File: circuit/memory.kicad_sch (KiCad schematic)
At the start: 26 parts, among them J2 Port C, J3 Port E, J4 Port A, J4 Port G, J5 Port D, U2 74HTC175

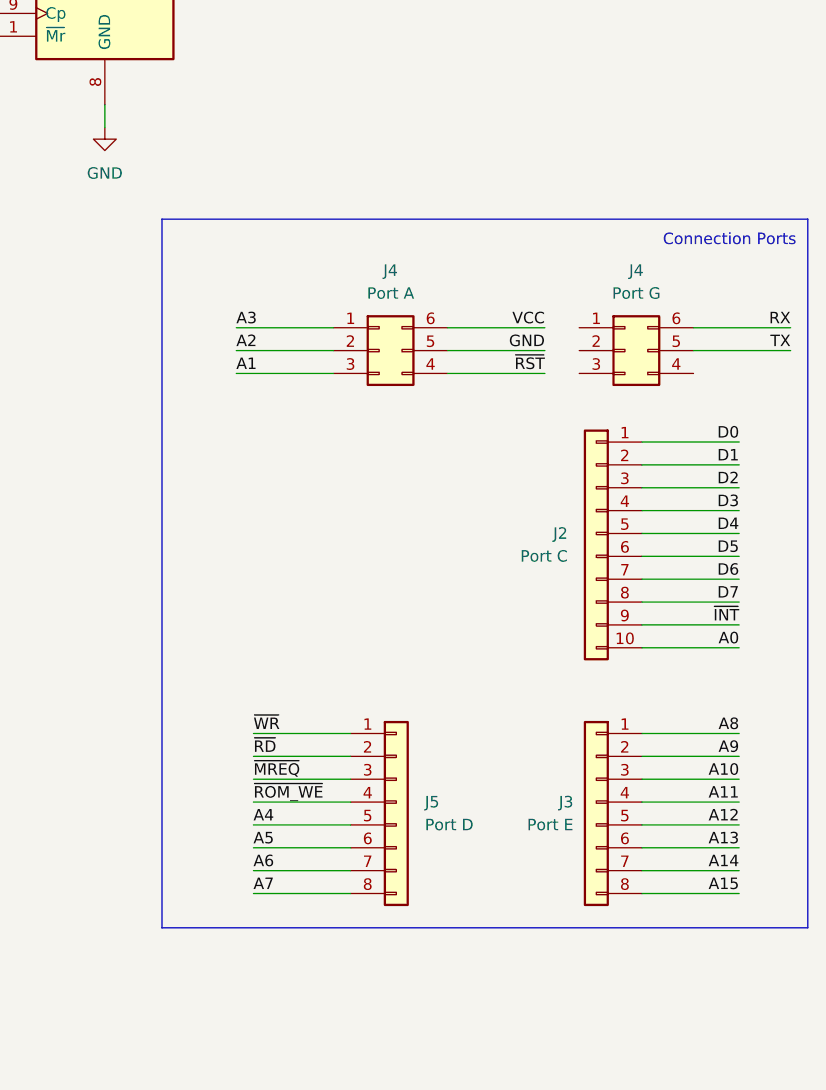
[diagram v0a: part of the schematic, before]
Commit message: .
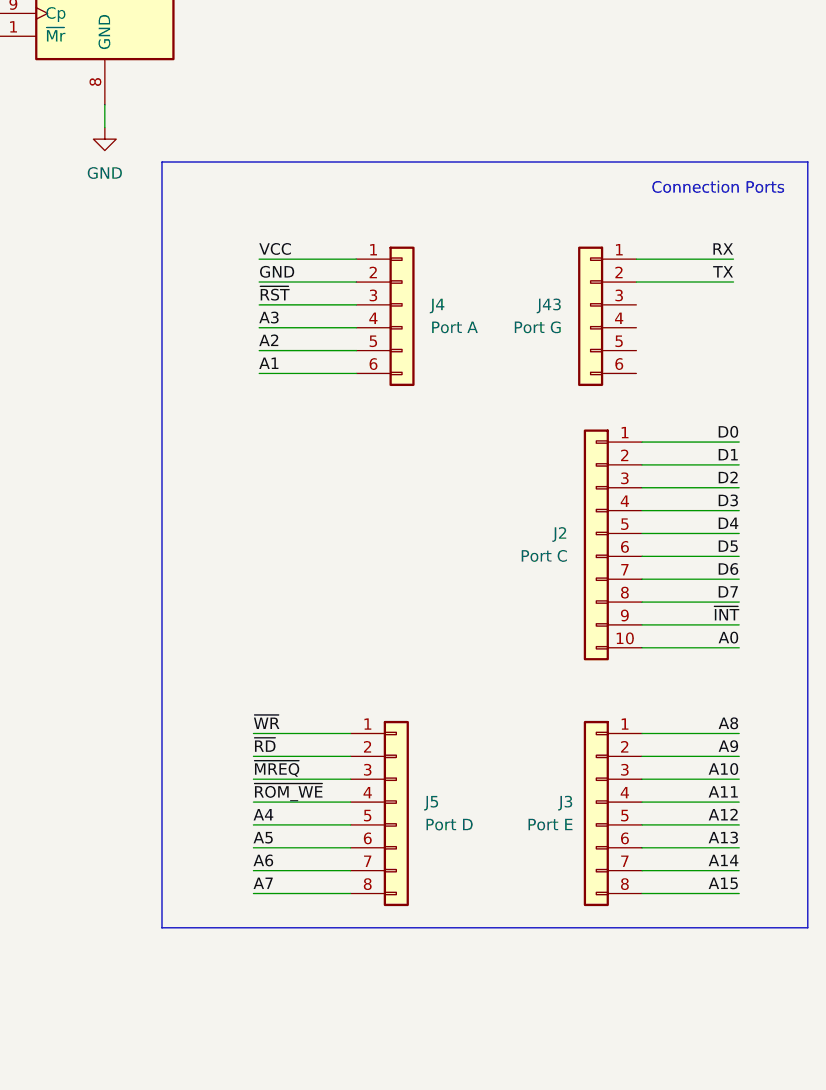
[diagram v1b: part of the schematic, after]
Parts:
- removed J4: Port A, symbol Connector_Generic:Conn_02x03_Counter_Clockwise
- removed J4: Port G, symbol Connector_Generic:Conn_02x03_Counter_Clockwise
- added J4: Port A, symbol Connector_Generic:Conn_01x06
- added J43: Port G, symbol Connector_Generic:Conn_01x06
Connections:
- net A1: now also J4.6 (Pin_6)
- net A2: now also J4.5 (Pin_5)
- net A3: now also J4.4 (Pin_4)
- net GND: now also J4.2 (Pin_2)
- net RX: now also J43.1 (Pin_1)
- net TX: now also J43.2 (Pin_2)
- net VCC: now also J4.1 (Pin_1)
- net ~{RST}: now also J4.3 (Pin_3)
